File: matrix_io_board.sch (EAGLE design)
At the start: 101 parts, among them IC1 6N138, IC2 LM27675M5_CHARGEPUMP, IC3 LM324D, IC4 MCP4728_QUAD_DAC, IC5 4504D, IC6 74AHC1G14DBV, IC7 FDS8958B, IC8 SP34063A_BOOST_REG

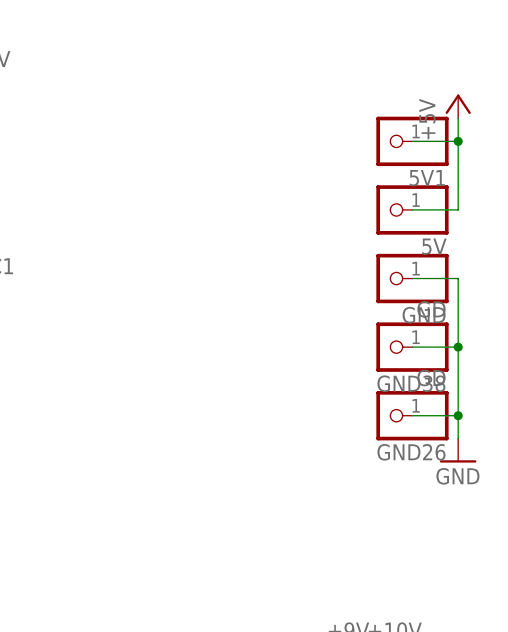
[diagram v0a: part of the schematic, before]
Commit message: rename
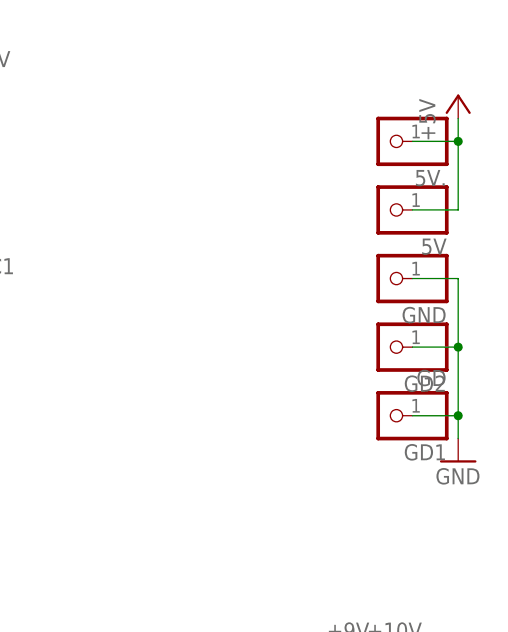
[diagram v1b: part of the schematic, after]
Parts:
- GD2: value GD -> (none)
- renumbered 5V1 to 5V., GND26 to GD1, GND38 to GD2
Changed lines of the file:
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@@
 <part name="P+15" library="supply1" deviceset="+5V" device=""/>
 <part name="GND30" library="supply1" deviceset="GND" device=""/>
-<part name="GND38" library="pinhead" deviceset="PINHD-1X1" device="" value="GD"/>
+<part name="GD2" library="pinhead" deviceset="PINHD-1X1" device=""/>
 <part name="GND40" library="supply1" deviceset="GND" device=""/>
 <part name="L1" library="SparkFun" deviceset="INDUCTOR" device="1210"/>
@@
 <part name="PWRCTL" library="pinhead" deviceset="PINHD-1X1" device=""/>
 <part name="AUX" library="microbuilder" deviceset="TESTPOINT" device="ROUND2MM"/>
-<part name="GND26" library="pinhead" deviceset="PINHD-1X1" device="" value="GD"/>
-<part name="5V1" library="pinhead" deviceset="PINHD-1X1" device=""/>
+<part name="GD1" library="pinhead" deviceset="PINHD-1X1" device="" value="GD"/>
+<part name="5V." library="pinhead" deviceset="PINHD-1X1" device=""/>
 <part name="OFFSW" library="pinhead" deviceset="PINHD-1X1" device=""/>
 </parts>
@@
 <instance part="P+15" gate="1" x="421.64" y="347.98"/>
 <instance part="GND30" gate="1" x="421.64" y="307.34"/>
-<instance part="GND38" gate="G$1" x="414.02" y="320.04" rot="R180"/>
+<instance part="GD2" gate="G$1" x="414.02" y="320.04" rot="R180"/>
 <instance part="GND40" gate="1" x="109.22" y="165.1"/>
 <instance part="L1" gate="G$1" x="271.78" y="317.5" rot="R90"/>
@@
 <instance part="PWRCTL" gate="G$1" x="99.06" y="330.2" rot="R180"/>
 <instance part="AUX" gate="G$1" x="388.62" y="228.6" rot="R180"/>
-<instance part="GND26" gate="G$1" x="414.02" y="312.42" rot="R180"/>
-<instance part="5V1" gate="G$1" x="414.02" y="342.9" rot="R180"/>
+<instance part="GD1" gate="G$1" x="414.02" y="312.42" rot="R180"/>
+<instance part="5V." gate="G$1" x="414.02" y="342.9" rot="R180"/>
 <instance part="OFFSW" gate="G$1" x="269.24" y="170.18"/>
 </instances>
@@
 <wire x1="416.56" y1="327.66" x2="421.64" y2="327.66" width="0.1524" layer="91"/>
 <wire x1="421.64" y1="327.66" x2="421.64" y2="320.04" width="0.1524" layer="91"/>
-<pinref part="GND38" gate="G$1" pin="1"/>
+<pinref part="GD2" gate="G$1" pin="1"/>
 <wire x1="421.64" y1="320.04" x2="421.64" y2="312.42" width="0.1524" layer="91"/>
 <wire x1="421.64" y1="312.42" x2="421.64" y2="309.88" width="0.1524" layer="91"/>
 <wire x1="416.56" y1="320.04" x2="421.64" y2="320.04" width="0.1524" layer="91"/>
 <junction x="421.64" y="320.04"/>
-<pinref part="GND26" gate="G$1" pin="1"/>
+<pinref part="GD1" gate="G$1" pin="1"/>
 <wire x1="416.56" y1="312.42" x2="421.64" y2="312.42" width="0.1524" layer="91"/>
 <junction x="421.64" y="312.42"/>
@@
 <wire x1="416.56" y1="335.28" x2="421.64" y2="335.28" width="0.1524" layer="91"/>
 <wire x1="421.64" y1="335.28" x2="421.64" y2="342.9" width="0.1524" layer="91"/>
-<pinref part="5V1" gate="G$1" pin="1"/>
+<pinref part="5V." gate="G$1" pin="1"/>
 <wire x1="421.64" y1="342.9" x2="421.64" y2="345.44" width="0.1524" layer="91"/>
 <wire x1="416.56" y1="342.9" x2="421.64" y2="342.9" width="0.1524" layer="91"/>

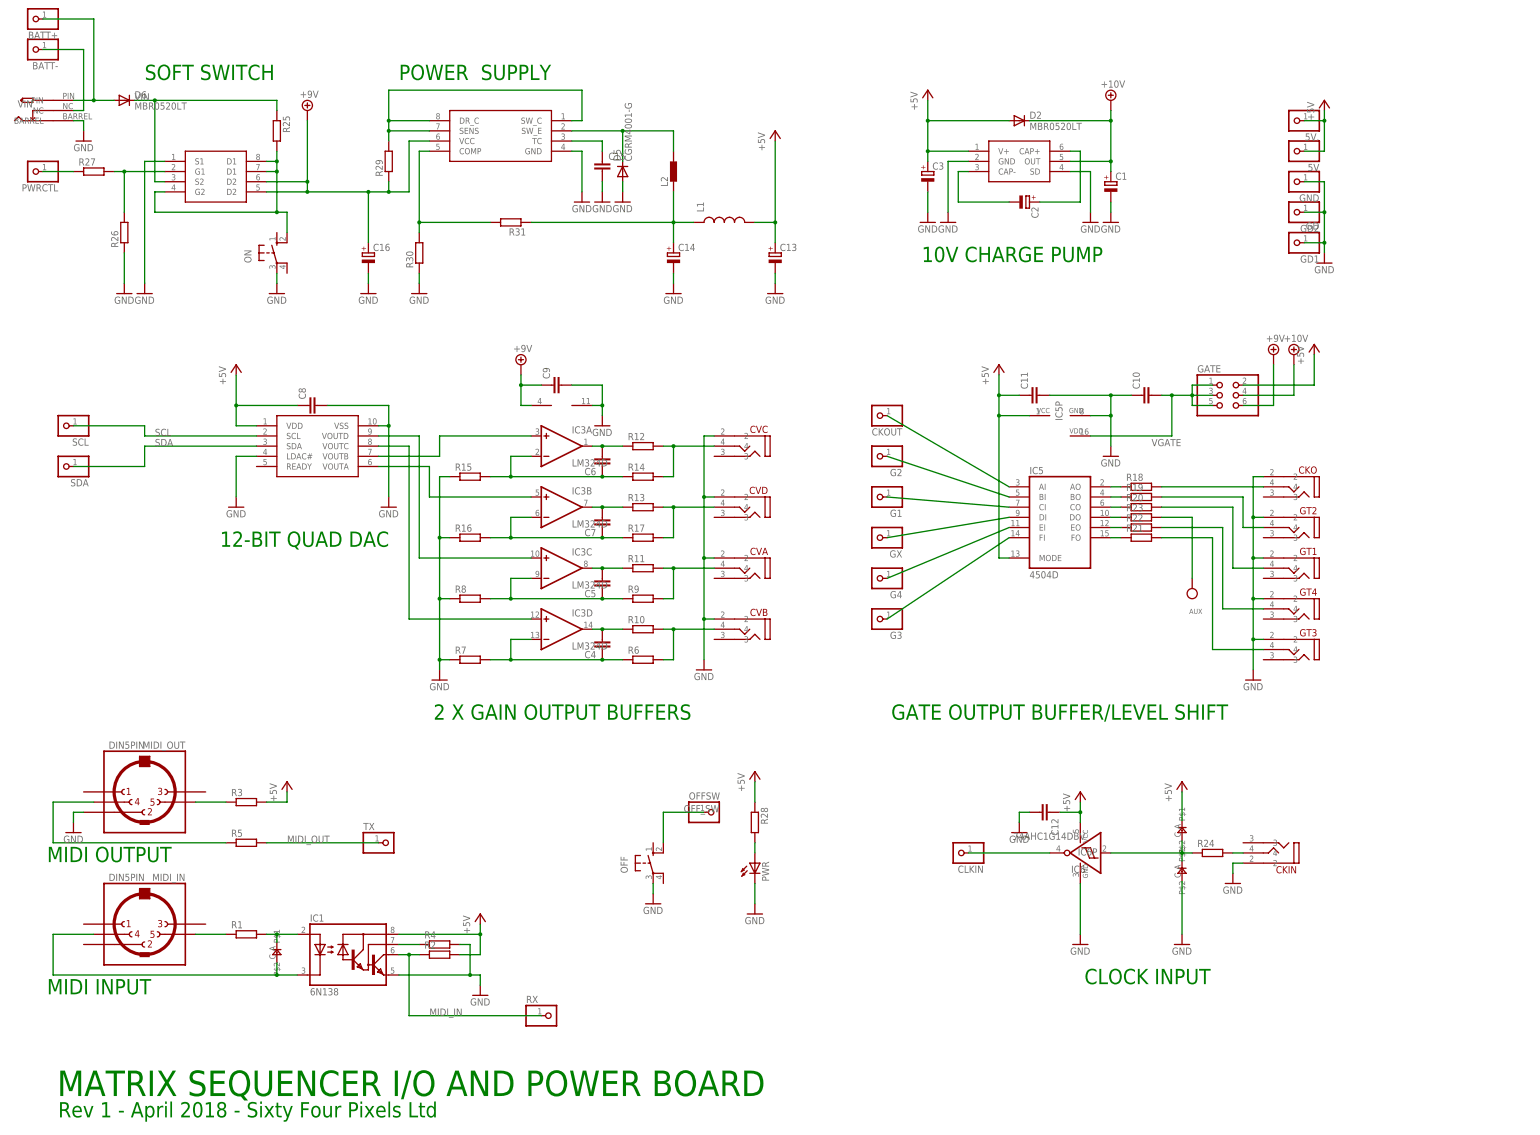
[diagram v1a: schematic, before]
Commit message: changes for rev2
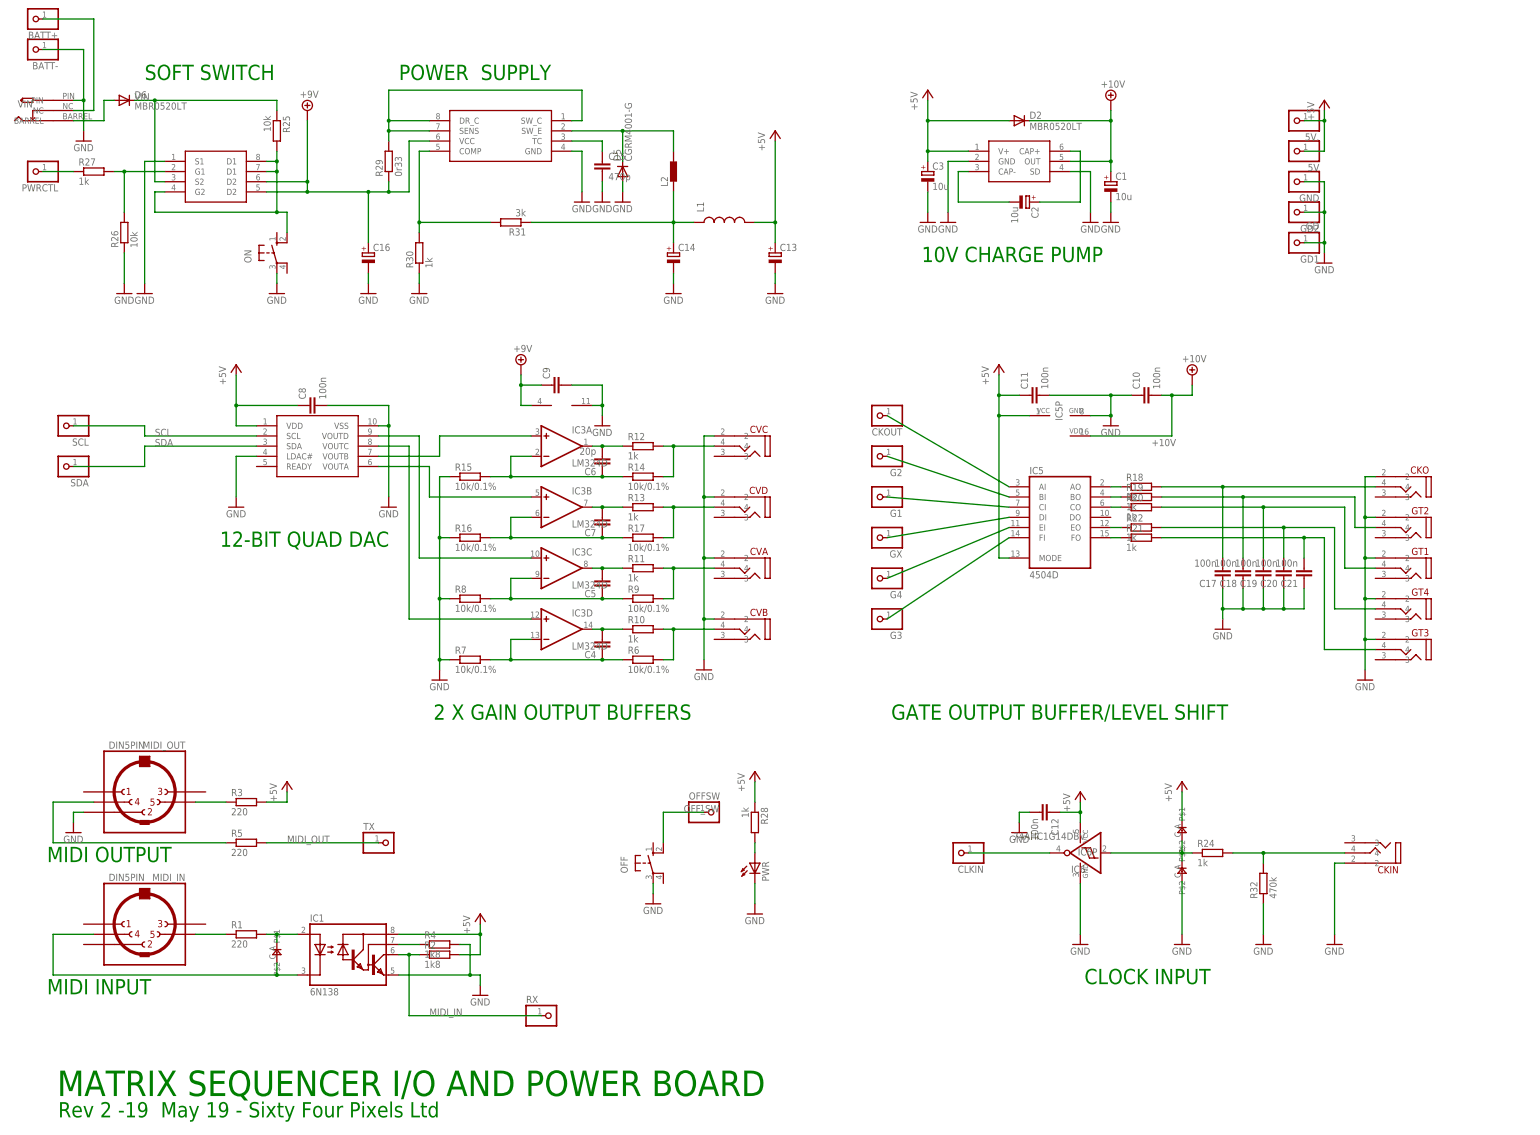
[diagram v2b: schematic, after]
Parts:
- removed AUX: (no value), microbuilder:TESTPOINTROUND2MM
- removed GATE: (no value), pinhead:PINHD-2X3
- removed R23: (no value), rcl:R-EU_R0805
- added C17, C18, C19, C20, C21: 100n, rcl:C-EUC0805
- added R32: 470k, rcl:R-EU_R0805
- C1, C2, C3: value (none) -> 10u
- C10, C11, C12, C8: value (none) -> 100n
- C15: value (none) -> 470p
- C6: value (none) -> 20p
- R1, R3, R5: value (none) -> 220
- R10, R11, R12, R13, R18, R19, R20, R21, R22, R24, R27, R28, R30: value (none) -> 1k
- R14, R15, R16, R17, R6, R7, R8, R9: value (none) -> 10k/0.1%
- R2, R4: value (none) -> 1k8
- R25, R26: value (none) -> 10k
- R29: value (none) -> 0r33
- R31: value (none) -> 3k
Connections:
- removed net N$42: IC5A.DO, R23.1
- removed net N$50: AUX.P$1, R23.2
- removed net N$71: BATT-.1, U$1.NC
- removed net VGATE: C10.2, GATE.1, GATE.3, GATE.5, IC5P.VDD
- new net N$16: BATT+.1, U$1.NC
- net +10V: now also C10.2, IC5P.VDD; no longer GATE.4
- net +5V: no longer GATE.2
- net +9V: no longer GATE.6
- net GND: now also BATT-.1, C17.1, C18.1, C19.1, C20.1, C21.1, R32.1, U$1.PIN; no longer U$1.BARREL
- net N$36: now also U$1.BARREL; no longer BATT+.1, U$1.PIN
- net N$44: now also C17.2
- net N$45: now also C18.2
- net N$46: now also C19.2
- net N$47: now also C20.2
- net N$48: now also C21.2
- net N$54: now also R32.2
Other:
- note added: "Rev 2 -19 May 19 - Sixty Four Pixels Ltd"
- note removed: "Rev 1 - April 2018 - Sixty Four Pixels Ltd"
- moved on the sheet: CKIN, CKO, GT1, GT2, GT3, GT4

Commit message: work in progress
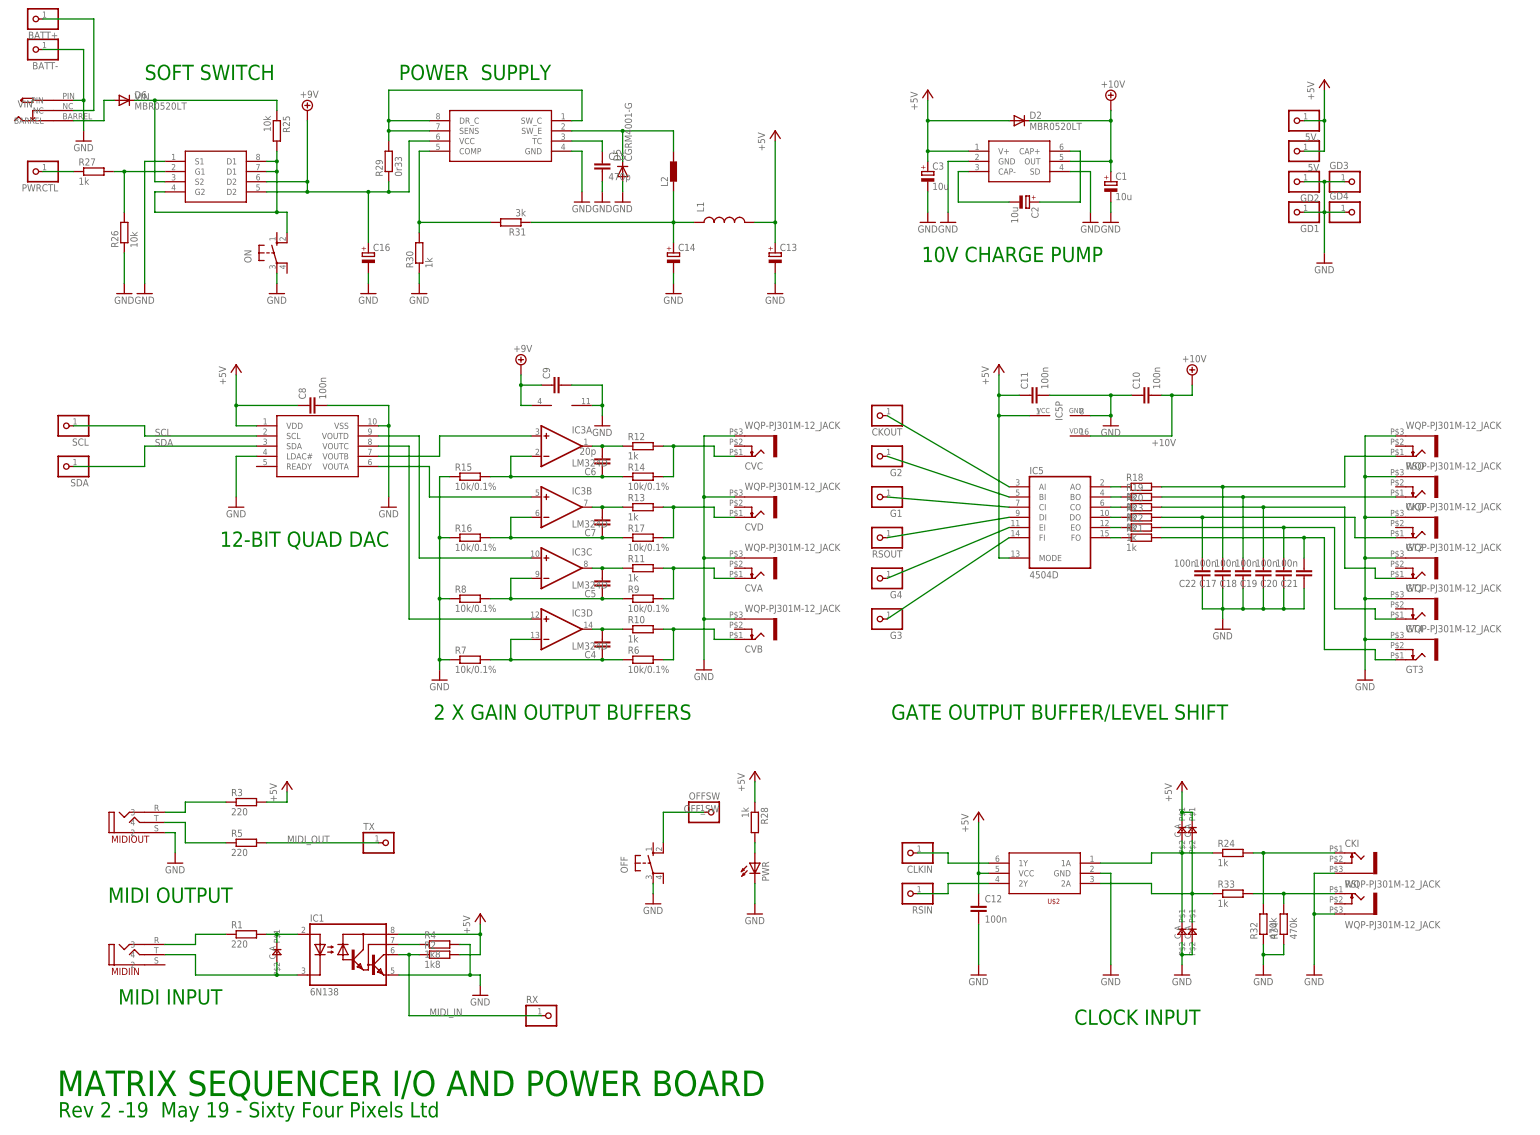
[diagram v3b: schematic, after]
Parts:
- removed CKIN: VERTICAL_3_5MM_SOCKET, jason_eagle6:VERTICAL_3_5MM_SOCKET
- removed GND: (no value), pinhead:PINHD-1X1
- removed IC6: 74AHC1G14DBV, 74xx-little-de:74AHC1G14DBV
- removed MIDI_IN, MIDI_OUT: DIN5PIN, jason_eagle6:DIN5PIN
- added C22: 100n, rcl:C-EUC0805
- added CKI, RSI, RSO: WQP-PJ301M-12_JACK, thonkiconn:WQP-PJ301M-12_JACK
- added D7, D8: 0805DIODE, jasons_stuff:0805DIODE
- added GD3, GD4, RSIN: (no value), pinhead:PINHD-1X1
- added MIDIIN, MIDIOUT: VERTICAL_3_5MM_SOCKETTHONK, jason_eagle6:VERTICAL_3_5MM_SOCKETTHONK
- added R23, R33: 1k, rcl:R-EU_R0805
- added R34: 470k, rcl:R-EU_R0805
- added U$2: SN74LVC2G14, jason_eagle6:SN74LVC2G14
- CKO, CVA, CVB, CVC, CVD, GT1, GT2, GT3, GT4: value VERTICAL_3_5MM_SOCKET -> WQP-PJ301M-12_JACK; device jason_eagle6:VERTICAL_3_5MM_SOCKET -> thonkiconn:WQP-PJ301M-12_JACK
- GD1: value GD -> (none)
- L2: device inductors:DR1030 -> jason_eagle6:NB_IND
- renumbered GX to RSOUT
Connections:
- removed net CLKIN: CLKIN.1, IC6A.O
- new net N$19: IC5A.DO, R23.1
- new net N$23: CLKIN.1, U$2.1Y
- new net N$24: R33.2, R34.2, RSI.2
- new net N$25: RSIN.1, U$2.2Y
- new net N$26: D7.P$1, D8.P$2, R33.1, U$2.2A
- new net N$27: C22.2, GT2.2, R23.2
- net +5V: now also D7.P$2, U$2.VCC; no longer IC6P.VCC
- net GND: now also C22.1, CKI.1, CKO.1, CVA.1, CVB.1, CVC.1, CVD.1, D8.P$1, GD3.1, GD4.1, GT1.1, GT2.1, GT3.1, GT4.1, MIDIOUT.2, R34.1, RSI.1, RSO.1, U$2.GND; no longer CKIN.2, CKO.2, CVA.2, CVB.2, CVC.2, CVD.2, GND.1, GT1.2, GT2.2, GT3.2, GT4.2, IC6P.GND, MIDI_OUT.2
- net N$1: now also MIDIOUT.3; no longer MIDI_OUT.5
- net N$10: now also CVB.2; no longer CVB.4
- net N$11: now also CVA.2; no longer CVA.4
- net N$4: now also MIDIIN.4; no longer MIDI_IN.4
- net N$44: now also RSO.2; no longer CKO.4
- net N$45: now also CKO.2; no longer GT2.4
- net N$46: now also GT1.2; no longer GT1.4
- net N$47: now also GT4.2; no longer GT4.4
- net N$48: now also GT3.2; no longer GT3.4
- net N$53: now also U$2.1A; no longer IC6A.I
- net N$54: now also CKI.2; no longer CKIN.4
- net N$6: now also MIDIOUT.4; no longer MIDI_OUT.4
- net N$7: now also MIDIIN.3; no longer MIDI_IN.5
- net N$8: now also CVC.2; no longer CVC.4
- net N$9: now also CVD.2; no longer CVD.4
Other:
- moved on the sheet: C12, CLKIN, GD1, GD2, R24, R32
